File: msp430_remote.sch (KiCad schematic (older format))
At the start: 10 parts

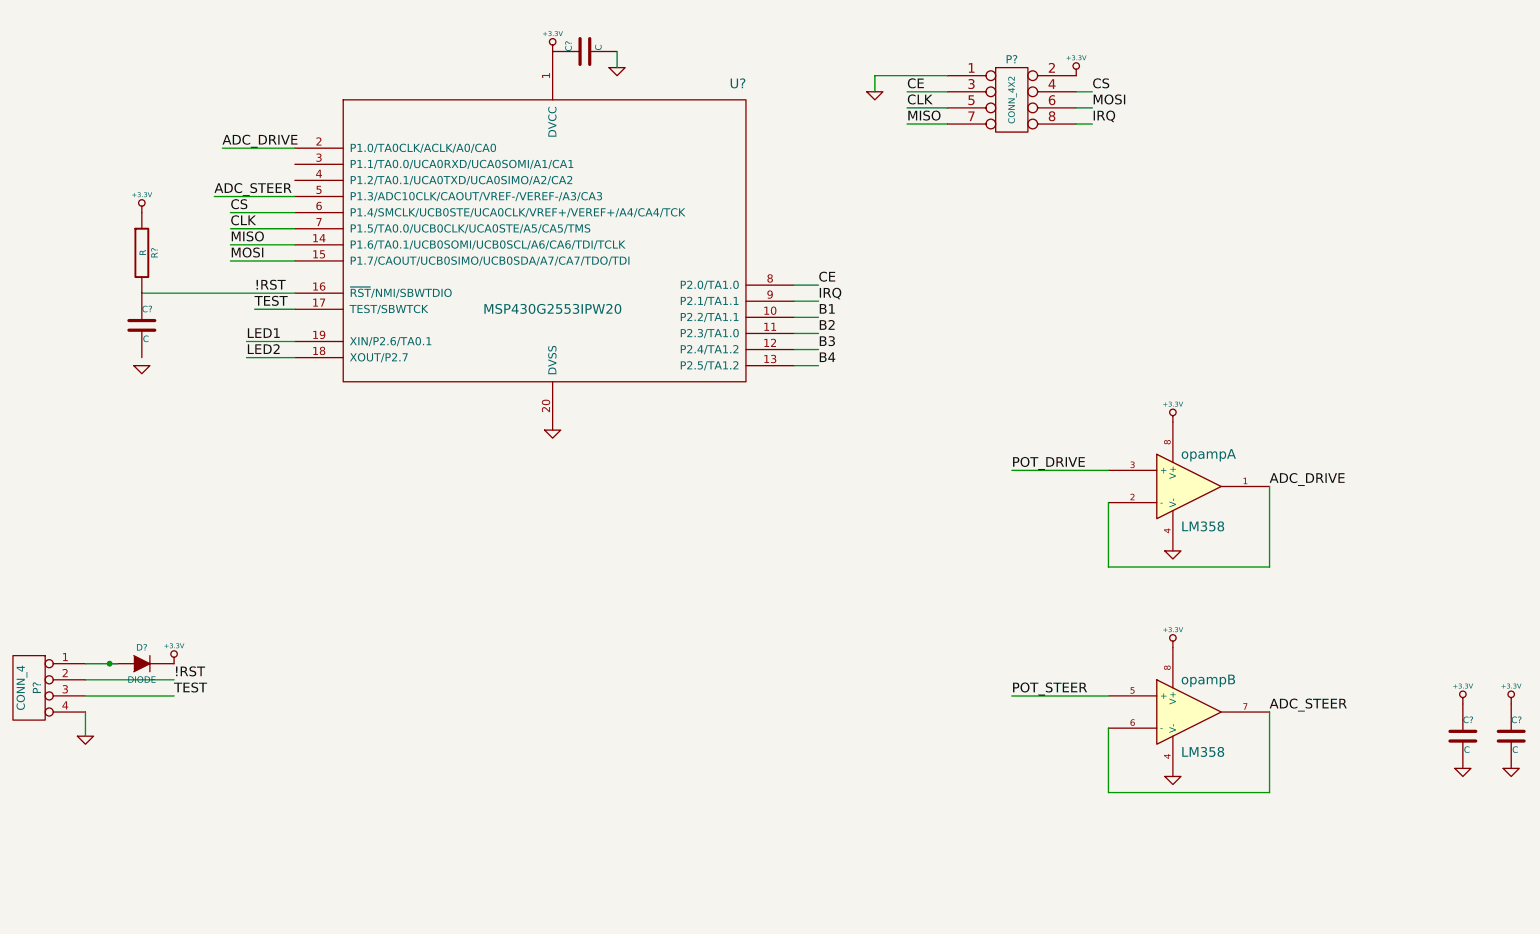
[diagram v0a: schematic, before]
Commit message: falta o dc dc
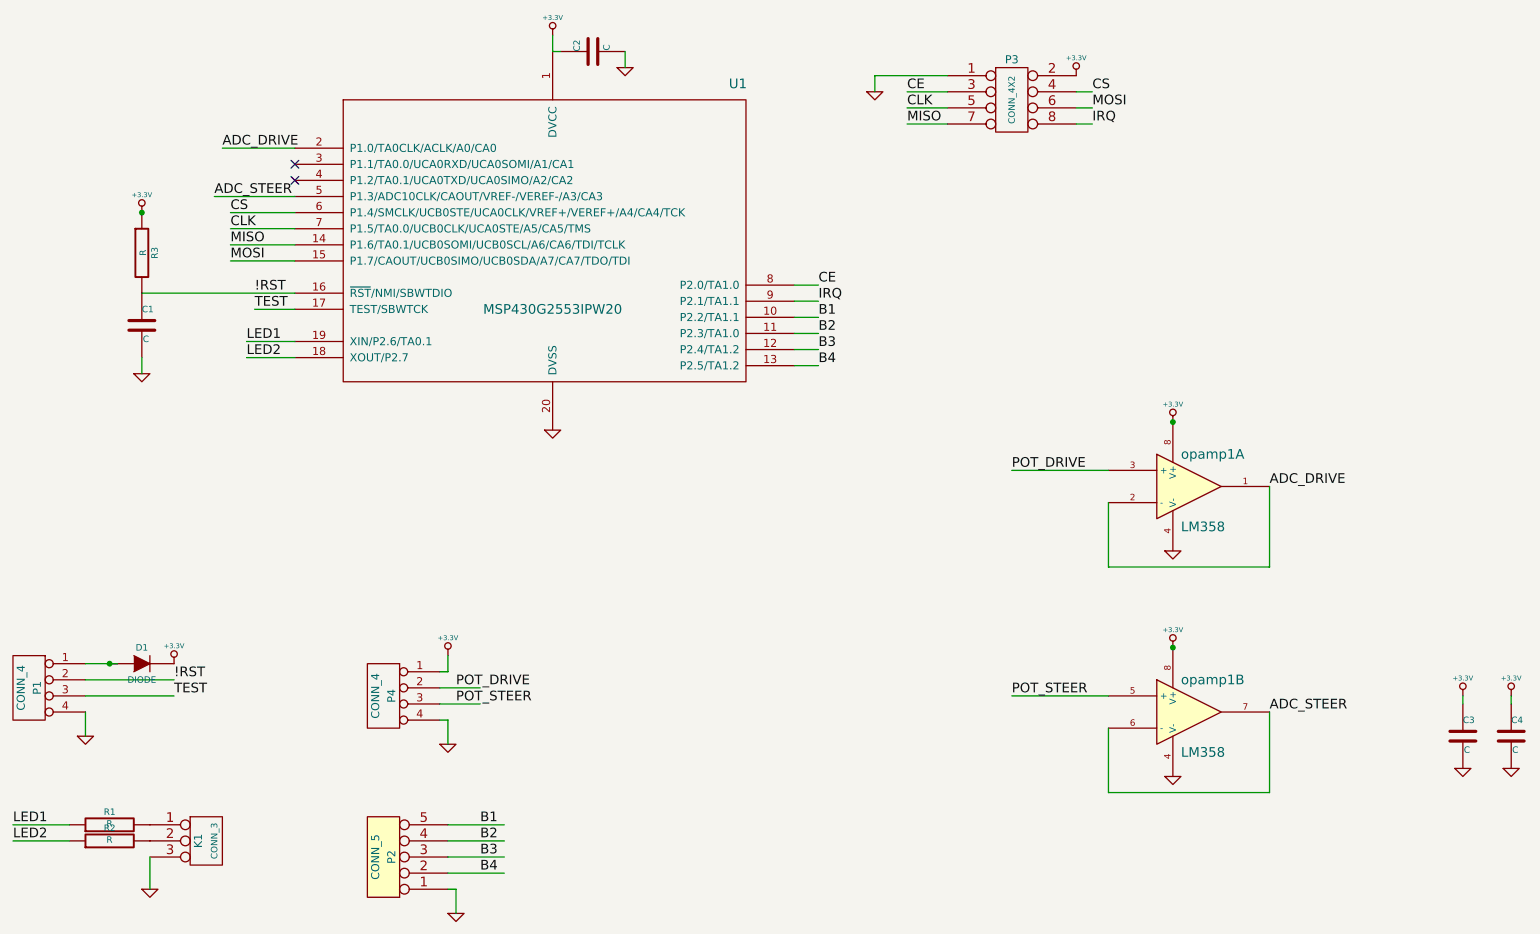
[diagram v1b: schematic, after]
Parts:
- added K1: CONN_3, ~, symbol CONN_3
- added P2: CONN_5, ~, symbol CONN_5
- added P4: CONN_4, ~, symbol CONN_4
- added R1, R2: R, ~, symbol R
- gave numbers to parts that had none: 9
- renumbered opamp to opamp1
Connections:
- wire segments 37 -> 57
- no-connect marks 0 -> 2
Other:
- moved on the sheet: C2
